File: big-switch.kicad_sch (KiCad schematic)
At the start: 7 parts, among them J1 Conn_01x07_Socket, SW1 SW_Push, SW2 RotaryEncoder_Switch, SW3 RotaryEncoder_Switch, U1 ProMicro

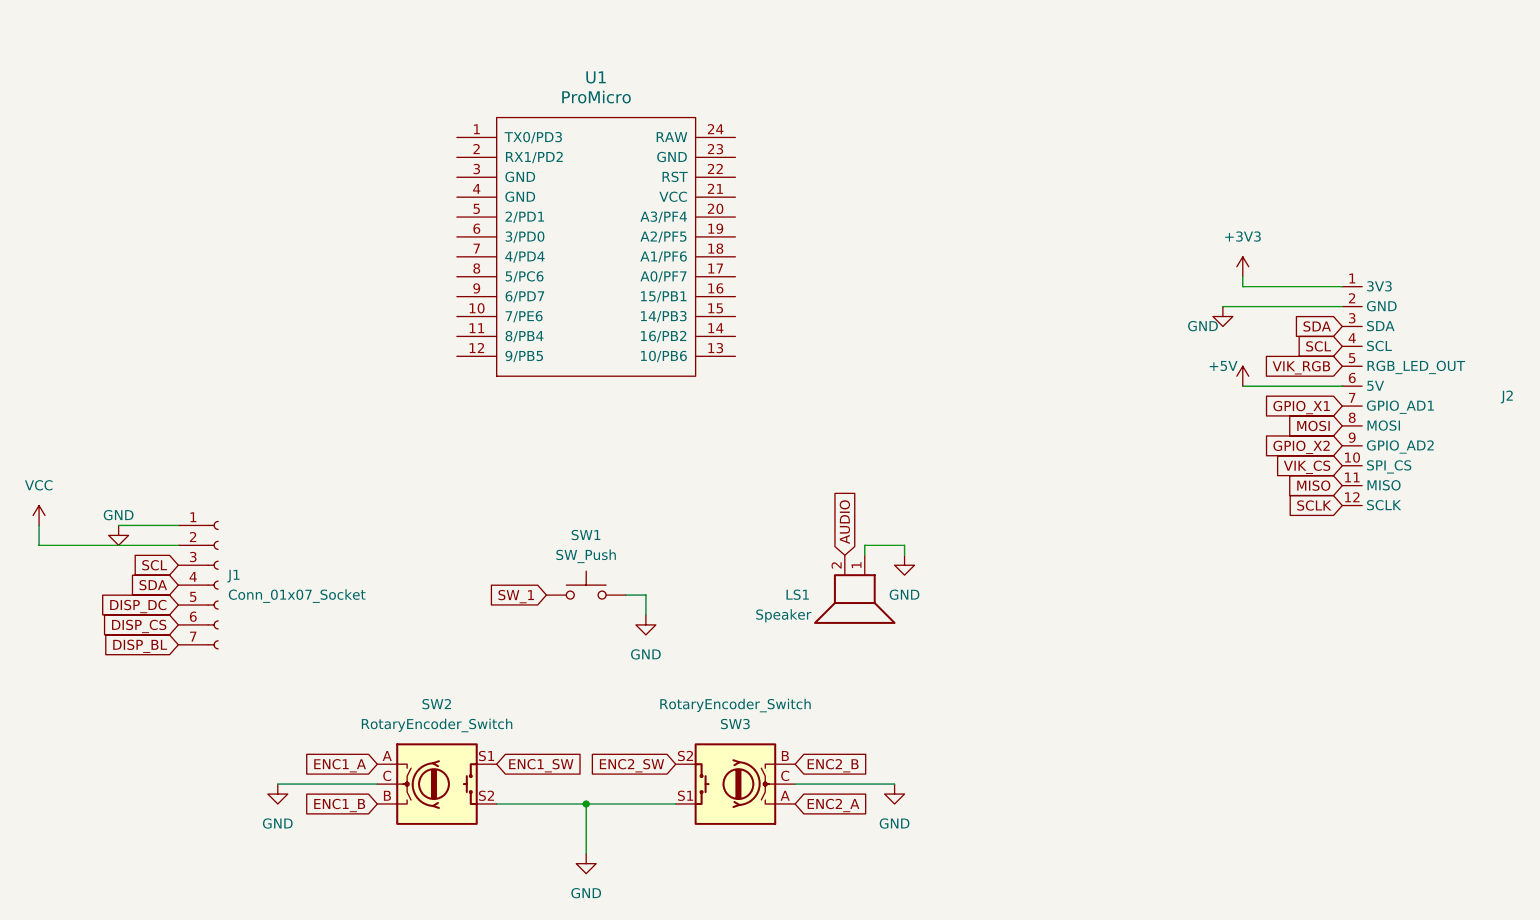
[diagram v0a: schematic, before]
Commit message: routing ocmplete
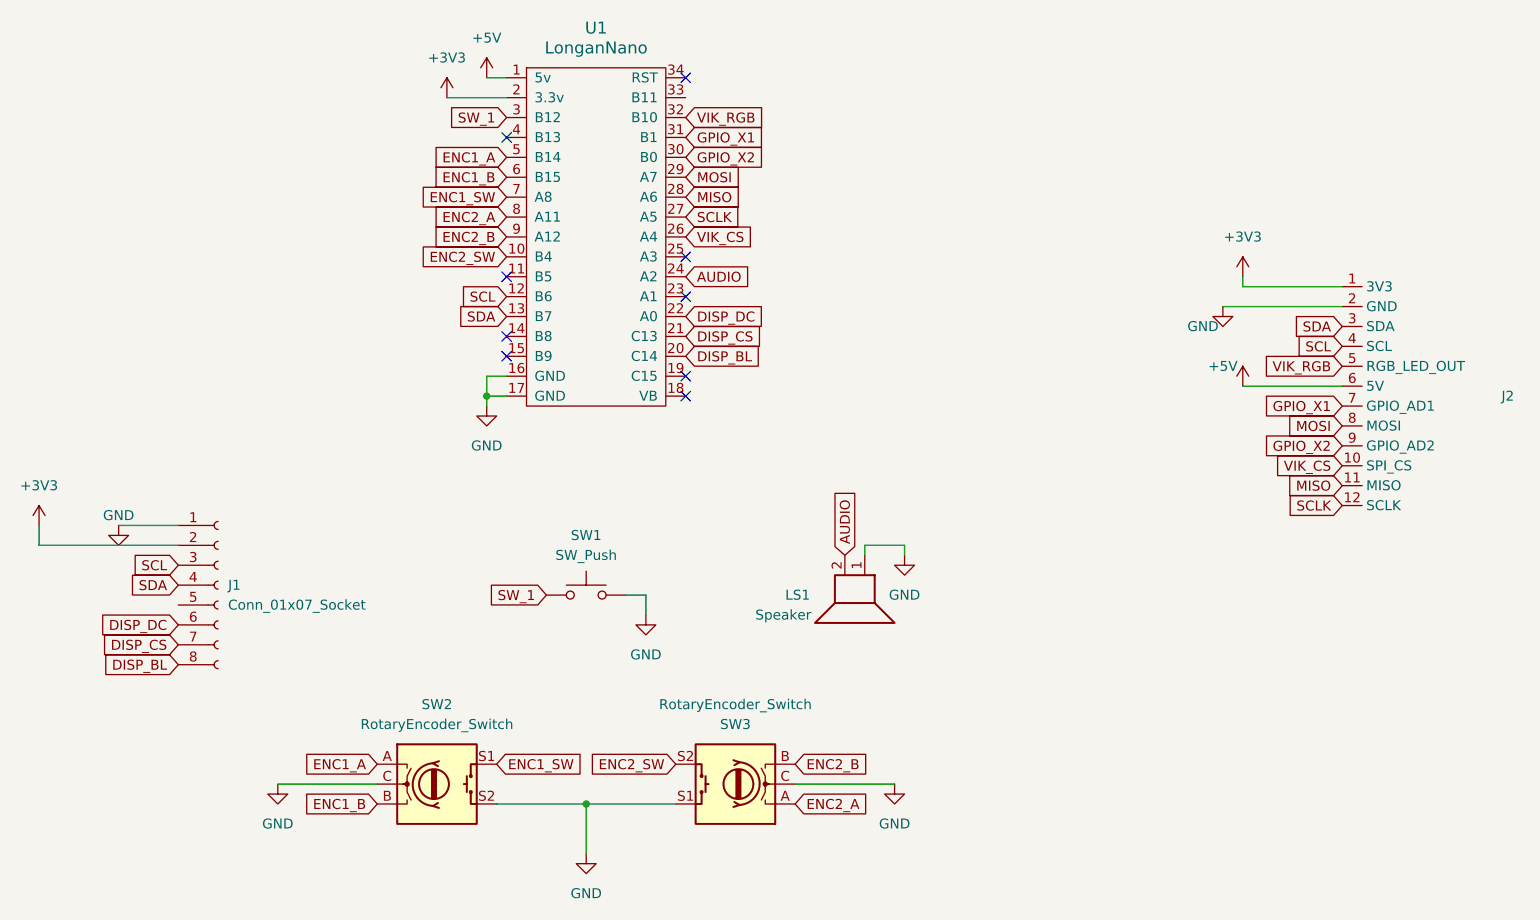
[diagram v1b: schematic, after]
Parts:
- J1: symbol Connector:Conn_01x07_Socket -> Connector:Conn_01x08_Socket
- SW2, SW3: footprint (none) -> Keebio-Parts:RotaryEncoder_EC11B-Horizontal-Dual
- U1: value ProMicro -> LonganNano; symbol keebio:ProMicro -> ws2812b:Longan_Nano
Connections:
- net VCC is gone; now on net +3V3: J1.2 (Pin_2)
- net +3V3: now also U1.2 (3.3v)
- net +5V: now also U1.1 (5v)
- net AUDIO: now also U1.24 (A2)
- net DISP_BL: now also J1.8 (Pin_8), U1.20 (C14); no longer J1.7 (Pin_7)
- net DISP_CS: now also J1.7 (Pin_7), U1.21 (C13); no longer J1.6 (Pin_6)
- net DISP_DC: now also J1.6 (Pin_6), U1.22 (A0); no longer J1.5 (Pin_5)
- net ENC1_A: now also U1.5 (B14)
- net ENC1_B: now also U1.6 (B15)
- net ENC1_SW: now also U1.7 (A8)
- net ENC2_A: now also U1.8 (A11)
- net ENC2_B: now also U1.9 (A12)
- net ENC2_SW: now also U1.10 (B4)
- net GND: now also U1.16 (GND), U1.17 (GND)
- net GPIO_X1: now also U1.31 (B1)
- net GPIO_X2: now also U1.30 (B0)
- net MISO: now also U1.28 (A6)
- net MOSI: now also U1.29 (A7)
- net SCL: now also U1.12 (B6)
- net SCLK: now also U1.27 (A5)
- net SDA: now also U1.13 (B7)
- net SW_1: now also U1.3 (B12)
- net VIK_CS: now also U1.26 (A4)
- net VIK_RGB: now also U1.32 (B10)
- no-connect marks 0 -> 9
